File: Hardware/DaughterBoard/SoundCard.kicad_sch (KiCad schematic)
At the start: 16 parts, among them J5 AUDIO_OUT, U1 ATmega328P-PU

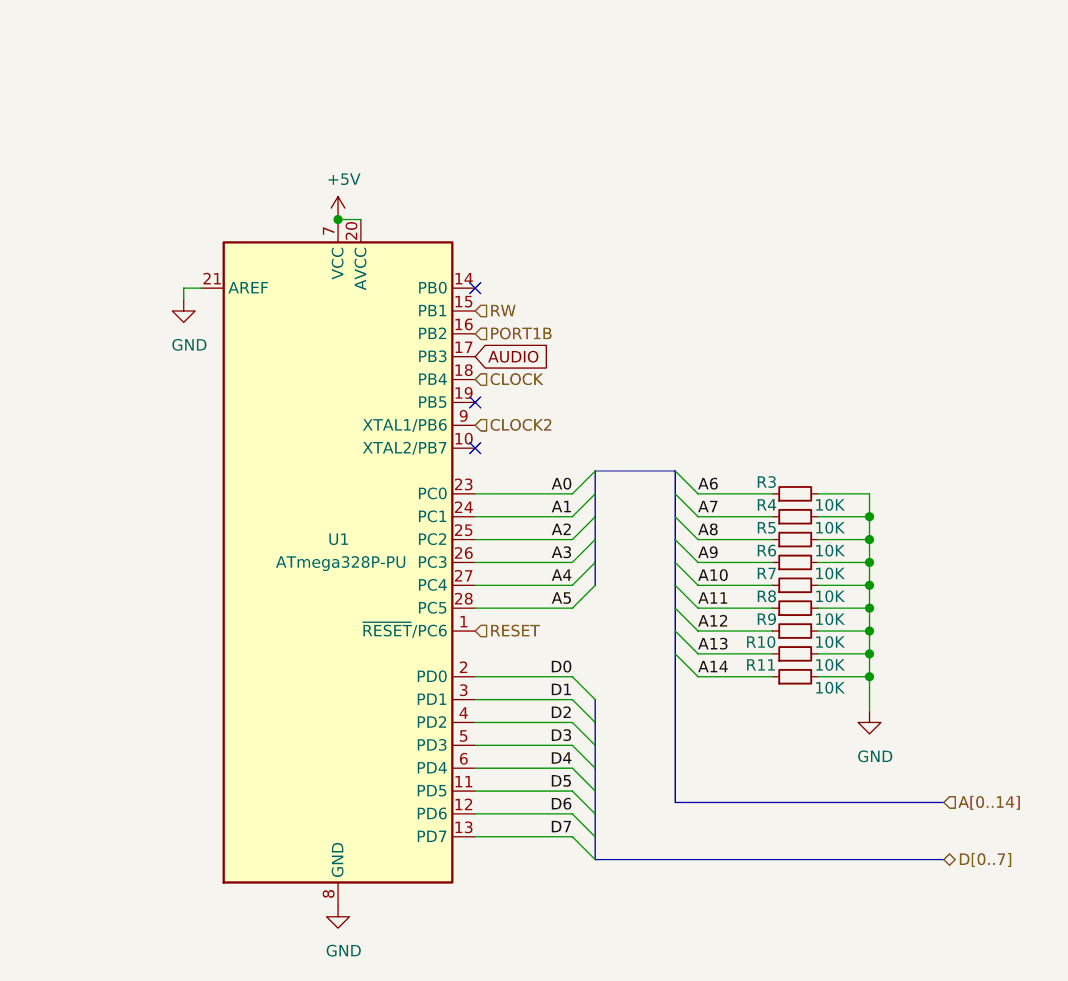
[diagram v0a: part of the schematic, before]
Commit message: Version 1.2
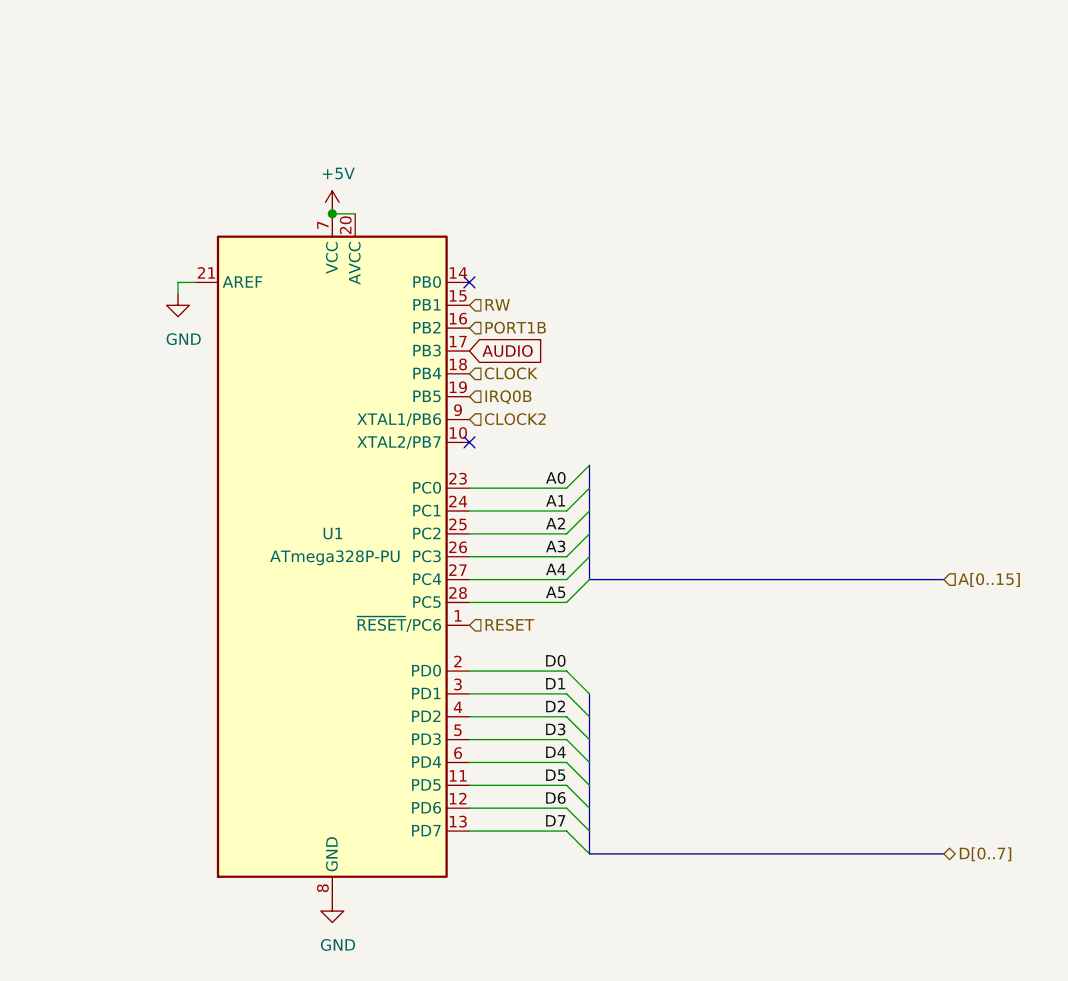
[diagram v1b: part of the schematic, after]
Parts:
- removed R10, R11, R3, R4, R5, R6, R7, R8, R9: 10K, Resistor_THT:R_Axial_DIN0207_L6.3mm_D2.5mm_P10.16mm_Horizontal, symbol Device:R_Small
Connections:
- net IRQ0B: now reaches U1.19 (PB5)
- no-connect marks 3 -> 2
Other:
- moved on the sheet: U1
